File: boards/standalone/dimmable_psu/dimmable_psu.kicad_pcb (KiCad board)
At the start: 2 copper layers, 78 parts, among them J1 DIM_IN, J2 PWM_IN, J3 POWER, J4 POWER_OUT, Q1 2N7002, Q2 IRF540N, Q3 IRF540N, U1 LM324, U2 LMC7660, U3 TPS92640

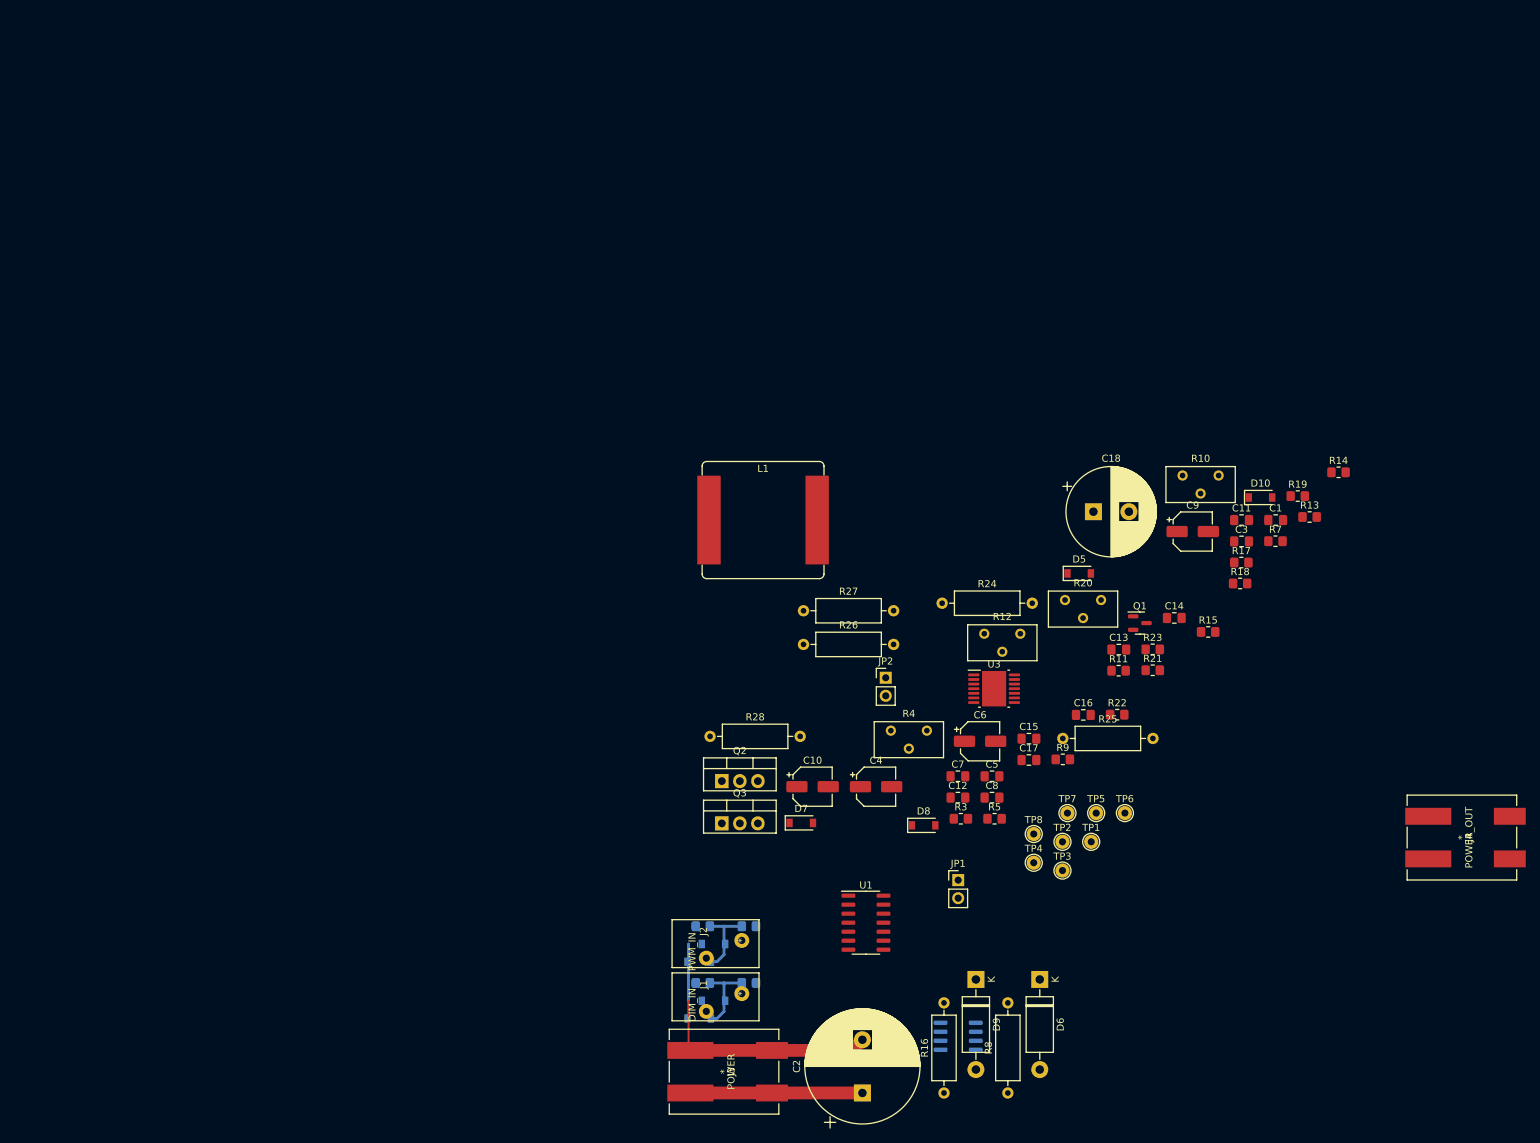
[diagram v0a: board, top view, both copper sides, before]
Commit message: mounting holes!
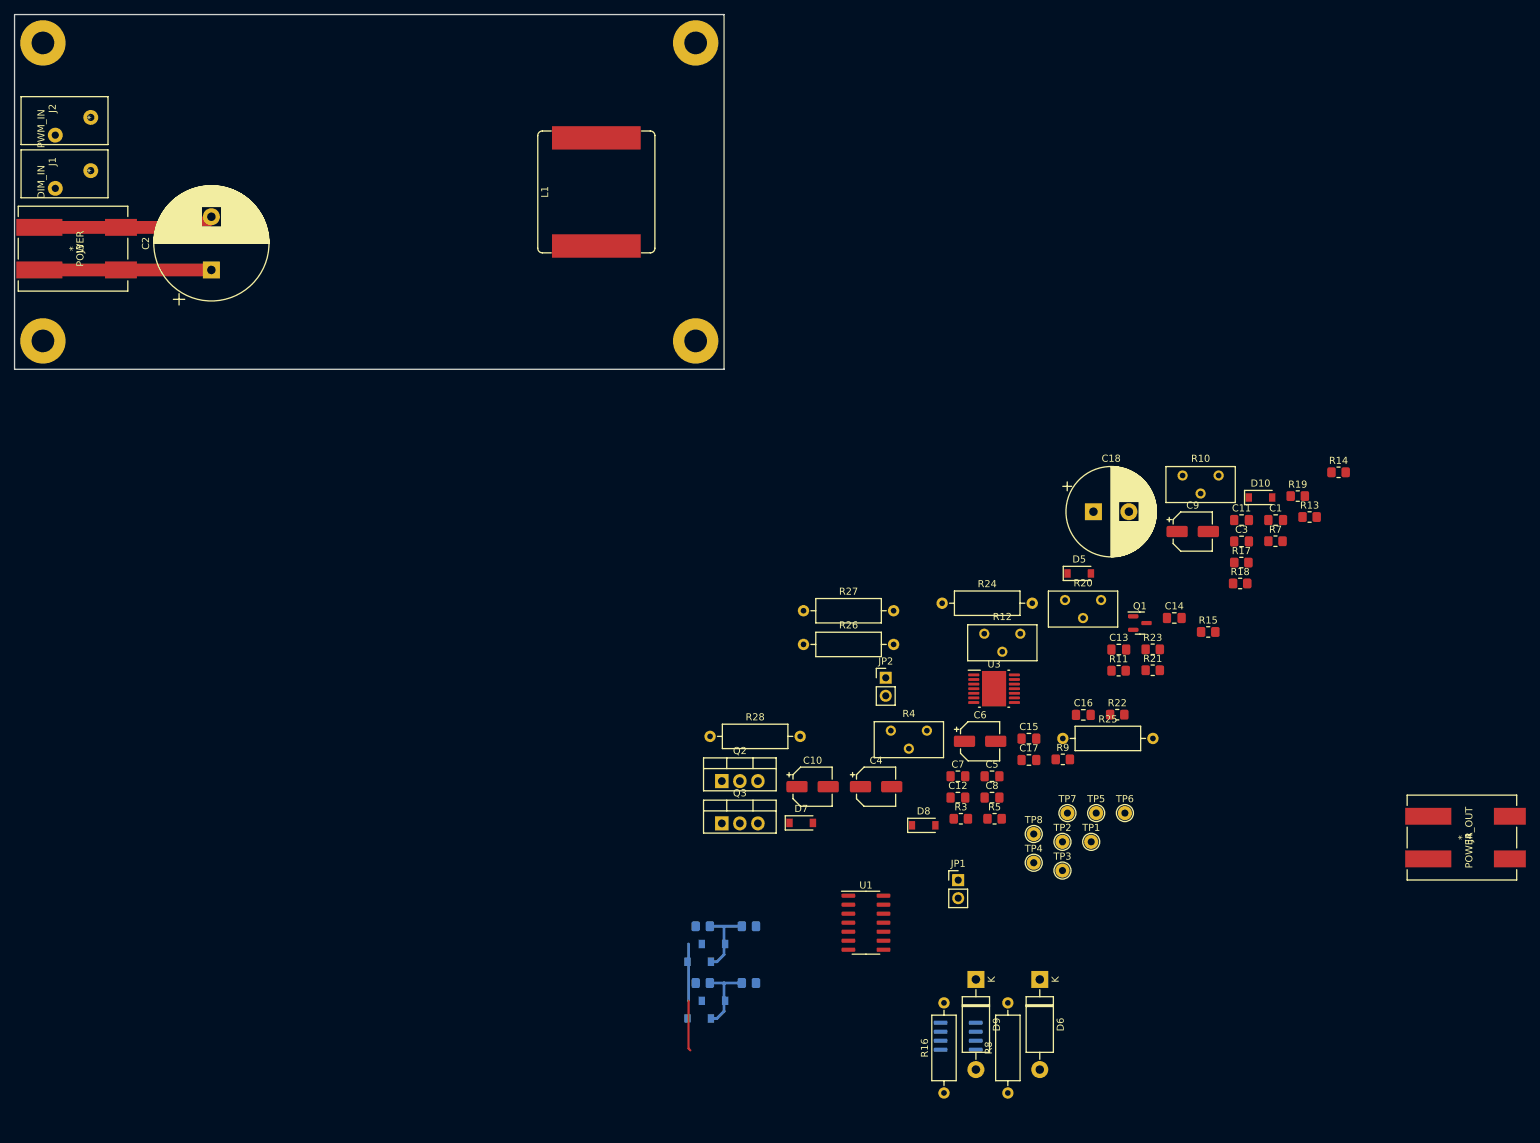
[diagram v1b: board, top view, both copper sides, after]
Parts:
- added H1: MountingHole_Pad, MountingHole:MountingHole_3.2mm_M3_Pad, F.Cu at (4.00, 4.00)
- added H2: MountingHole_Pad, MountingHole:MountingHole_3.2mm_M3_Pad, F.Cu at (96.0, 4.00)
- added H3: MountingHole_Pad, MountingHole:MountingHole_3.2mm_M3_Pad, F.Cu at (96.0, 46.0)
- added H4: MountingHole_Pad, MountingHole:MountingHole_3.2mm_M3_Pad, F.Cu at (4.00, 46.0)
- moved C2 147.9 mm to (27.7, 36.0)
- moved J1 147.9 mm to (10.7, 22.0)
- moved J2 147.9 mm to (10.7, 14.5)
- moved J3 147.9 mm to (8.24, 33.0)
- moved L1 51.9 mm to (82.0, 25.0), turned to 90 degrees
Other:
- board outline added: 100 x 50 mm
